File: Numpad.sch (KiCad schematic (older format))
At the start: 50 parts, among them SW1 SW_Push, U1 ATmega32U4-AU, Y1 16MHz

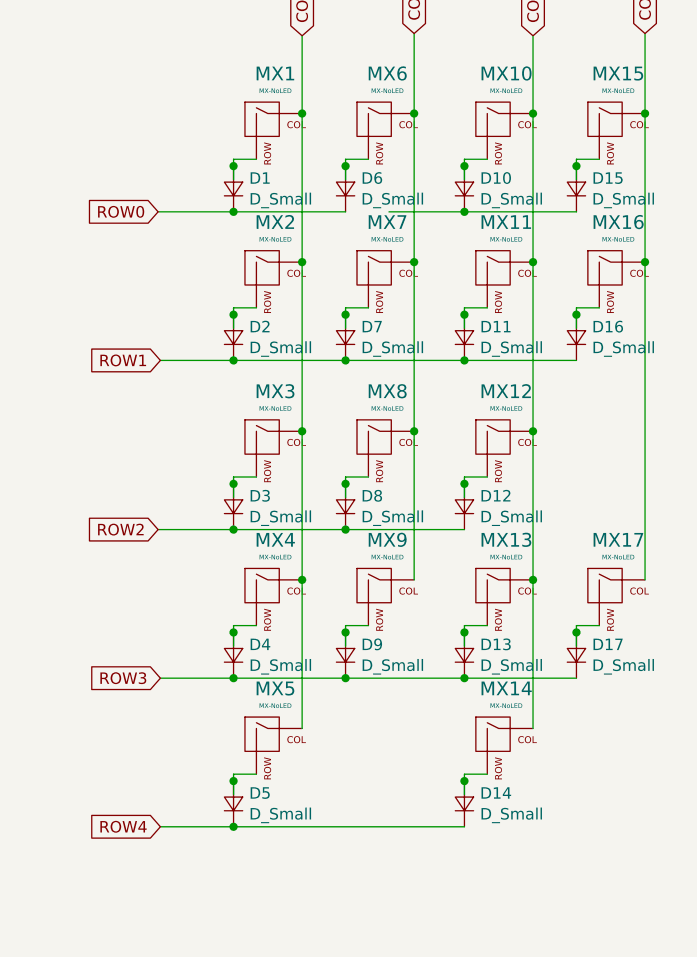
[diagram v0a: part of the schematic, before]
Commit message: Save progress
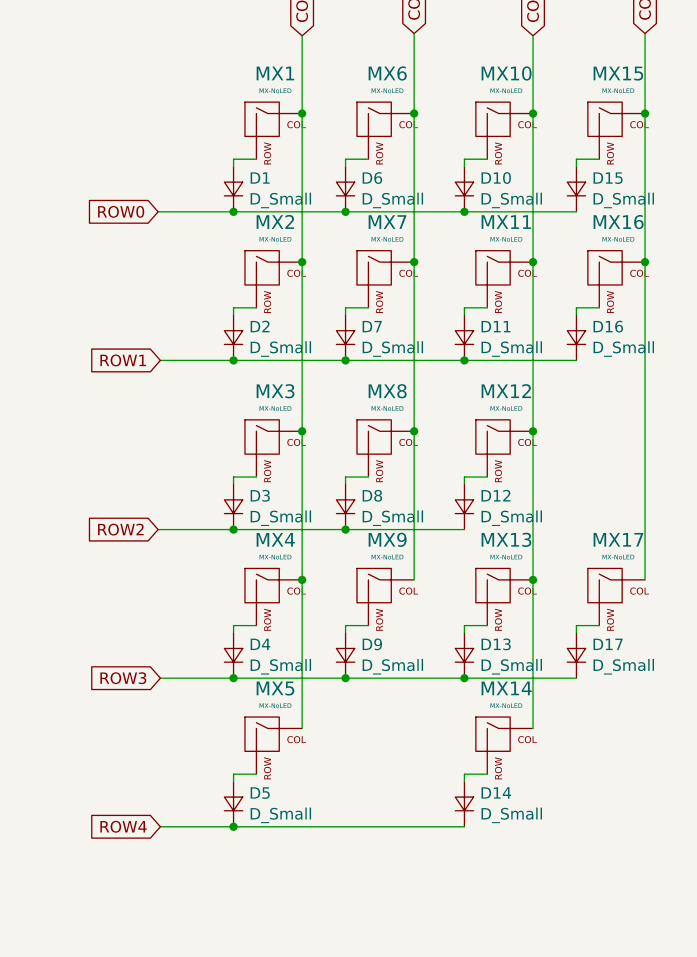
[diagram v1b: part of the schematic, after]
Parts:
- MX1, MX10, MX11, MX12, MX13, MX14, MX15, MX2, MX3, MX4, MX6, MX7, MX8, MX9: footprint (none) -> MX_Alps_Hybrid:MX-1U-NoLED
- MX16, MX17, MX5: footprint (none) -> MX_Alps_Hybrid:MX-2U-NoLED
- R1, R2, R3, R4: footprint (none) -> Resistor_SMD:R_0805_2012Metric
- SW1: footprint (none) -> random-keyboard-parts:SKQG-1155865
- USB1: footprint (none) -> random-keyboard-parts:Molex-0548190589
- Y1: footprint (none) -> Crystal:Crystal_SMD_3225-4Pin_3.2x2.5mm
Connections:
- wire segments 140 -> 123
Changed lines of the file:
@@
 F 0 "R4" V 4234 5010 50  0000 C CNN
 F 1 "10k" V 4325 5010 50  0000 C CNN
-F 2 "" H 4430 5010 50  0001 C CNN
+F 2 "Resistor_SMD:R_0805_2012Metric" H 4430 5010 50  0001 C CNN
 F 3 "~" H 4430 5010 50  0001 C CNN
 	1    4430 5010
@@
 F 0 "R1" V 2200 3850 50  0000 C CNN
 F 1 "22" V 2270 3850 50  0000 C CNN
-F 2 "" H 2270 3850 50  0001 C CNN
+F 2 "Resistor_SMD:R_0805_2012Metric" H 2270 3850 50  0001 C CNN
 F 3 "~" H 2270 3850 50  0001 C CNN
 	1    2270 3850
@@
 F 0 "R2" V 2340 3950 50  0000 C CNN
 F 1 "22" V 2270 3950 50  0000 C CNN
-F 2 "" H 2270 3950 50  0001 C CNN
+F 2 "Resistor_SMD:R_0805_2012Metric" H 2270 3950 50  0001 C CNN
 F 3 "~" H 2270 3950 50  0001 C CNN
 	1    2270 3950
@@
 F 0 "Y1" V 2226 3006 50  0000 R CNN
 F 1 "16MHz" V 2135 3006 50  0000 R CNN
-F 2 "" H 2180 3150 50  0001 C CNN
+F 2 "Crystal:Crystal_SMD_3225-4Pin_3.2x2.5mm" H 2180 3150 50  0001 C CNN
 F 3 "~" H 2180 3150 50  0001 C CNN
 	1    2180 3150
@@
 F 0 "SW1" H 2330 3135 50  0000 C CNN
 F 1 "SW_Push" H 2330 3044 50  0000 C CNN
-F 2 "" H 2330 3050 50  0001 C CNN
+F 2 "random-keyboard-parts:SKQG-1155865" H 2330 3050 50  0001 C CNN
 F 3 "~" H 2330 3050 50  0001 C CNN
 	1    2330 2850
@@
 F 0 "R3" H 2629 2596 50  0000 L CNN
 F 1 "10k" H 2629 2505 50  0000 L CNN
-F 2 "" H 2570 2550 50  0001 C CNN
+F 2 "Resistor_SMD:R_0805_2012Metric" H 2570 2550 50  0001 C CNN
 F 3 "~" H 2570 2550 50  0001 C CNN
 	1    2570 2550
@@
 F 0 "USB1" V 1607 1167 60  0000 C CNN
 F 1 "Molex-0548190589" V 1501 1167 60  0000 C CNN
-F 2 "" H 1070 1200 60  0001 C CNN
+F 2 "random-keyboard-parts:Molex-0548190589" H 1070 1200 60  0001 C CNN
 F 3 "" H 1070 1200 60  0001 C CNN
 	1    1070 1200
@@
 F 0 "MX1" H 7473 2703 60  0000 C CNN
 F 1 "MX-NoLED" H 7473 2629 20  0000 C CNN
-F 2 "" H 6815 2455 60  0001 C CNN
+F 2 "MX_Alps_Hybrid:MX-1U-NoLED" H 6815 2455 60  0001 C CNN
 F 3 "" H 6815 2455 60  0001 C CNN
 	1    7440 2480
@@
 $EndComp
 Wire Wire Line
-	7290 2720 7290 2660
-Wire Wire Line
 	7290 2630 7390 2630
-Connection ~ 7290 2660
 Wire Wire Line
 	7290 2660 7290 2630
@@
 F 0 "MX6" H 7963 2703 60  0000 C CNN
 F 1 "MX-NoLED" H 7963 2629 20  0000 C CNN
-F 2 "" H 7305 2455 60  0001 C CNN
+F 2 "MX_Alps_Hybrid:MX-1U-NoLED" H 7305 2455 60  0001 C CNN
 F 3 "" H 7305 2455 60  0001 C CNN
 	1    7930 2480
@@
 $EndComp
 Wire Wire Line
-	7780 2720 7780 2660
-Wire Wire Line
 	7780 2630 7880 2630
-Connection ~ 7780 2660
 Wire Wire Line
 	7780 2660 7780 2630
@@
 F 0 "MX2" H 7473 3353 60  0000 C CNN
 F 1 "MX-NoLED" H 7473 3279 20  0000 C CNN
-F 2 "" H 6815 3105 60  0001 C CNN
+F 2 "MX_Alps_Hybrid:MX-1U-NoLED" H 6815 3105 60  0001 C CNN
 F 3 "" H 6815 3105 60  0001 C CNN
 	1    7440 3130
@@
 $EndComp
 Wire Wire Line
-	7290 3370 7290 3310
-Wire Wire Line
 	7290 3280 7390 3280
-Connection ~ 7290 3310
 Wire Wire Line
 	7290 3310 7290 3280
@@
 F 0 "MX7" H 7963 3353 60  0000 C CNN
 F 1 "MX-NoLED" H 7963 3279 20  0000 C CNN
-F 2 "" H 7305 3105 60  0001 C CNN
+F 2 "MX_Alps_Hybrid:MX-1U-NoLED" H 7305 3105 60  0001 C CNN
 F 3 "" H 7305 3105 60  0001 C CNN
 	1    7930 3130
@@
 $EndComp
 Wire Wire Line
-	7780 3370 7780 3310
-Wire Wire Line
 	7780 3280 7880 3280
-Connection ~ 7780 3310
-Wire Wire Line
-	7780 3310 7780 3280
 Wire Wire Line
 	7290 2860 7780 2860
@@
 F 0 "MX10" H 8483 2703 60  0000 C CNN
 F 1 "MX-NoLED" H 8483 2629 20  0000 C CNN
-F 2 "" H 7825 2455 60  0001 C CNN
+F 2 "MX_Alps_Hybrid:MX-1U-NoLED" H 7825 2455 60  0001 C CNN
 F 3 "" H 7825 2455 60  0001 C CNN
 	1    8450 2480
@@
 	0    -1   -1   0
 $EndComp
-Wire Wire Line
-	8300 2720 8300 2660
-Wire Wire Line
-	8300 2630 8400 2630
-Connection ~ 8300 2660
-Wire Wire Line
-	8300 2660 8300 2630
 $Comp
 L MX_Alps_Hybrid:MX-NoLED MX15
@@
 F 0 "MX15" H 8973 2703 60  0000 C CNN
 F 1 "MX-NoLED" H 8973 2629 20  0000 C CNN
-F 2 "" H 8315 2455 60  0001 C CNN
+F 2 "MX_Alps_Hybrid:MX-1U-NoLED" H 8315 2455 60  0001 C CNN
 F 3 "" H 8315 2455 60  0001 C CNN
 	1    8940 2480
@@
 $EndComp
 Wire Wire Line
-	8790 2720 8790 2660
-Wire Wire Line
 	8790 2630 8890 2630
-Connection ~ 8790 2660
 Wire Wire Line
 	8790 2660 8790 2630
@@
 F 0 "MX11" H 8483 3353 60  0000 C CNN
 F 1 "MX-NoLED" H 8483 3279 20  0000 C CNN
-F 2 "" H 7825 3105 60  0001 C CNN
+F 2 "MX_Alps_Hybrid:MX-1U-NoLED" H 7825 3105 60  0001 C CNN
 F 3 "" H 7825 3105 60  0001 C CNN
 	1    8450 3130
@@
 $EndComp
 Wire Wire Line
-	8300 3370 8300 3310
-Wire Wire Line
 	8300 3280 8400 3280
-Connection ~ 8300 3310
 Wire Wire Line
 	8300 3310 8300 3280
@@
 F 0 "MX16" H 8973 3353 60  0000 C CNN
 F 1 "MX-NoLED" H 8973 3279 20  0000 C CNN
-F 2 "" H 8315 3105 60  0001 C CNN
+F 2 "MX_Alps_Hybrid:MX-2U-NoLED" H 8315 3105 60  0001 C CNN
 F 3 "" H 8315 3105 60  0001 C CNN
 	1    8940 3130
@@
 $EndComp
 Wire Wire Line
-	8790 3370 8790 3310
-Wire Wire Line
 	8790 3280 8890 3280
-Connection ~ 8790 3310
-Wire Wire Line
-	8790 3310 8790 3280
 Wire Wire Line
 	8300 2860 8790 2860
@@
 	9090 2430 9090 2080
 Connection ~ 9090 2430
-Wire Wire Line
-	8300 2860 7970 2860
 Connection ~ 8300 2860
 Connection ~ 8300 3510
@@
 F 0 "MX3" H 7473 4093 60  0000 C CNN
 F 1 "MX-NoLED" H 7473 4019 20  0000 C CNN
-F 2 "" H 6815 3845 60  0001 C CNN
+F 2 "MX_Alps_Hybrid:MX-1U-NoLED" H 6815 3845 60  0001 C CNN
 F 3 "" H 6815 3845 60  0001 C CNN
 	1    7440 3870
@@
 $EndComp
 Wire Wire Line
-	7290 4110 7290 4050
-Wire Wire Line
 	7290 4020 7390 4020
-Connection ~ 7290 4050
 Wire Wire Line
 	7290 4050 7290 4020
@@
 F 0 "MX8" H 7963 4093 60  0000 C CNN
 F 1 "MX-NoLED" H 7963 4019 20  0000 C CNN
-F 2 "" H 7305 3845 60  0001 C CNN
+F 2 "MX_Alps_Hybrid:MX-1U-NoLED" H 7305 3845 60  0001 C CNN
 F 3 "" H 7305 3845 60  0001 C CNN
 	1    7930 3870
@@
 $EndComp
 Wire Wire Line
-	7780 4110 7780 4050
-Wire Wire Line
 	7780 4020 7880 4020
-Connection ~ 7780 4050
-Wire Wire Line
-	7780 4050 7780 4020
 $Comp
 L MX_Alps_Hybrid:MX-NoLED MX4
@@
 F 0 "MX4" H 7473 4743 60  0000 C CNN
 F 1 "MX-NoLED" H 7473 4669 20  0000 C CNN
-F 2 "" H 6815 4495 60  0001 C CNN
+F 2 "MX_Alps_Hybrid:MX-1U-NoLED" H 6815 4495 60  0001 C CNN
 F 3 "" H 6815 4495 60  0001 C CNN
 	1    7440 4520
@@
 $EndComp
 Wire Wire Line
-	7290 4760 7290 4700
-Wire Wire Line
 	7290 4670 7390 4670
-Connection ~ 7290 4700
 Wire Wire Line
 	7290 4700 7290 4670
@@
 F 0 "MX9" H 7963 4743 60  0000 C CNN
 F 1 "MX-NoLED" H 7963 4669 20  0000 C CNN
-F 2 "" H 7305 4495 60  0001 C CNN
+F 2 "MX_Alps_Hybrid:MX-1U-NoLED" H 7305 4495 60  0001 C CNN
 F 3 "" H 7305 4495 60  0001 C CNN
 	1    7930 4520
@@
 $EndComp
 Wire Wire Line
-	7780 4760 7780 4700
-Wire Wire Line
 	7780 4670 7880 4670
-Connection ~ 7780 4700
-Wire Wire Line
-	7780 4700 7780 4670
 Wire Wire Line
 	7290 4250 7780 4250
@@
 F 0 "MX12" H 8483 4093 60  0000 C CNN
 F 1 "MX-NoLED" H 8483 4019 20  0000 C CNN
-F 2 "" H 7825 3845 60  0001 C CNN
+F 2 "MX_Alps_Hybrid:MX-1U-NoLED" H 7825 3845 60  0001 C CNN
 F 3 "" H 7825 3845 60  0001 C CNN
 	1    8450 3870
@@
 $EndComp
 Wire Wire Line
-	8300 4110 8300 4050
-Wire Wire Line
 	8300 4020 8400 4020
-Connection ~ 8300 4050
-Wire Wire Line
-	8300 4050 8300 4020
 $Comp
 L MX_Alps_Hybrid:MX-NoLED MX13
@@
 F 0 "MX13" H 8483 4743 60  0000 C CNN
 F 1 "MX-NoLED" H 8483 4669 20  0000 C CNN
-F 2 "" H 7825 4495 60  0001 C CNN
+F 2 "MX_Alps_Hybrid:MX-1U-NoLED" H 7825 4495 60  0001 C CNN
 F 3 "" H 7825 4495 60  0001 C CNN
 	1    8450 4520
@@
 $EndComp
 Wire Wire Line
-	8300 4760 8300 4700
-Wire Wire Line
 	8300 4670 8400 4670
-Connection ~ 8300 4700
 Wire Wire Line
 	8300 4700 8300 4670
@@
 $EndComp
 Wire Wire Line
-	8790 4760 8790 4700
-Connection ~ 8790 4700
-Wire Wire Line
 	8790 4700 8790 4670
 Wire Wire Line
@@
 F 0 "MX5" H 7473 5393 60  0000 C CNN
 F 1 "MX-NoLED" H 7473 5319 20  0000 C CNN
-F 2 "" H 6815 5145 60  0001 C CNN
+F 2 "MX_Alps_Hybrid:MX-2U-NoLED" H 6815 5145 60  0001 C CNN
 F 3 "" H 6815 5145 60  0001 C CNN
 	1    7440 5170
@@
 $EndComp
 Wire Wire Line
-	7290 5410 7290 5350
-Wire Wire Line
 	7290 5320 7390 5320
-Connection ~ 7290 5350
-Wire Wire Line
-	7290 5350 7290 5320
 Wire Wire Line
 	7590 4470 7590 5120
@@
 F 0 "MX14" H 8483 5393 60  0000 C CNN
 F 1 "MX-NoLED" H 8483 5319 20  0000 C CNN
-F 2 "" H 7825 5145 60  0001 C CNN
+F 2 "MX_Alps_Hybrid:MX-1U-NoLED" H 7825 5145 60  0001 C CNN
 F 3 "" H 7825 5145 60  0001 C CNN
 	1    8450 5170
@@
 $EndComp
 Wire Wire Line
-	8300 5410 8300 5350
-Wire Wire Line
 	8300 5320 8400 5320
-Connection ~ 8300 5350
-Wire Wire Line
-	8300 5350 8300 5320
 Wire Wire Line
 	8600 4470 8600 5120
@@
 F 0 "MX17" H 8973 4743 60  0000 C CNN
 F 1 "MX-NoLED" H 8973 4669 20  0000 C CNN
-F 2 "" H 8315 4495 60  0001 C CNN
+F 2 "MX_Alps_Hybrid:MX-2U-NoLED" H 8315 4495 60  0001 C CNN
 F 3 "" H 8315 4495 60  0001 C CNN
 	1    8940 4520
@@
 Wire Wire Line
 	1720 2970 1720 3250
+Wire Wire Line
+	8300 2660 8300 2630
+Wire Wire Line
+	8300 2630 8400 2630
+Wire Wire Line
+	8790 3280 8790 3310
+Wire Wire Line
+	7780 3280 7780 3310
+Wire Wire Line
+	7780 4020 7780 4050
+Wire Wire Line
+	8300 4020 8300 4050
+Wire Wire Line
+	7780 4670 7780 4700
+Wire Wire Line
+	7290 5320 7290 5350
+Wire Wire Line
+	8300 5350 8300 5320
+Wire Wire Line
+	7780 2860 8300 2860
+Connection ~ 7780 2860
 $EndSCHEMATC
